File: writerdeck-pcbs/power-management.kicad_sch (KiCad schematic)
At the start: 36 parts, among them J1 5000mAh 3.7V LiPo, J3 5000mAh 3.7V LiPo, U2 BQ25792RQMR

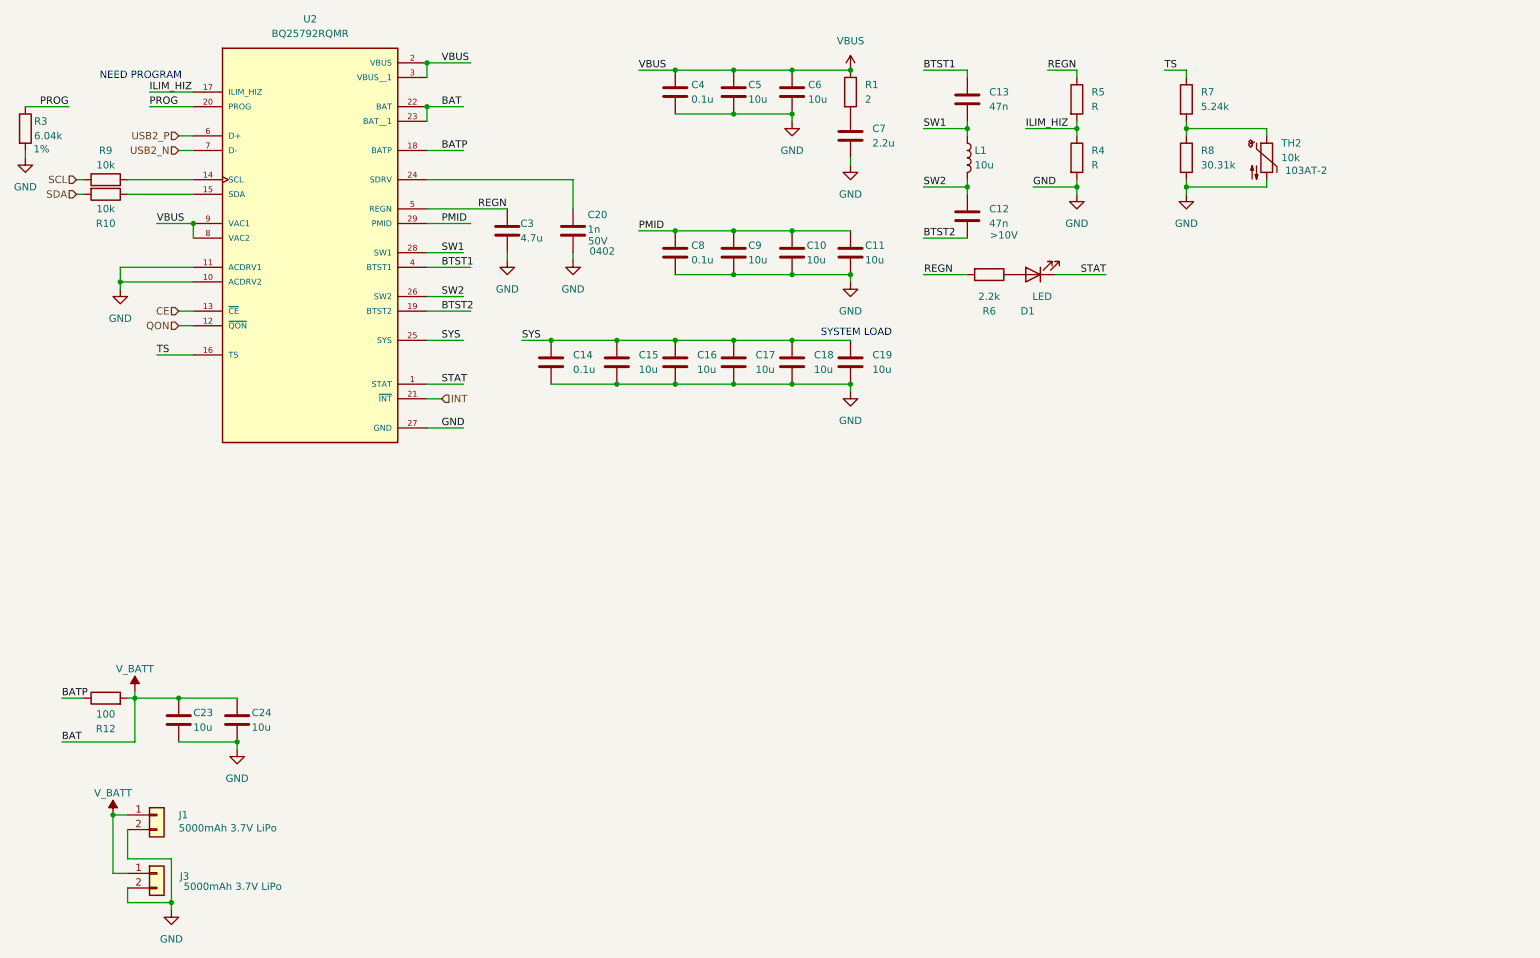
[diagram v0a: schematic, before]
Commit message: power management done
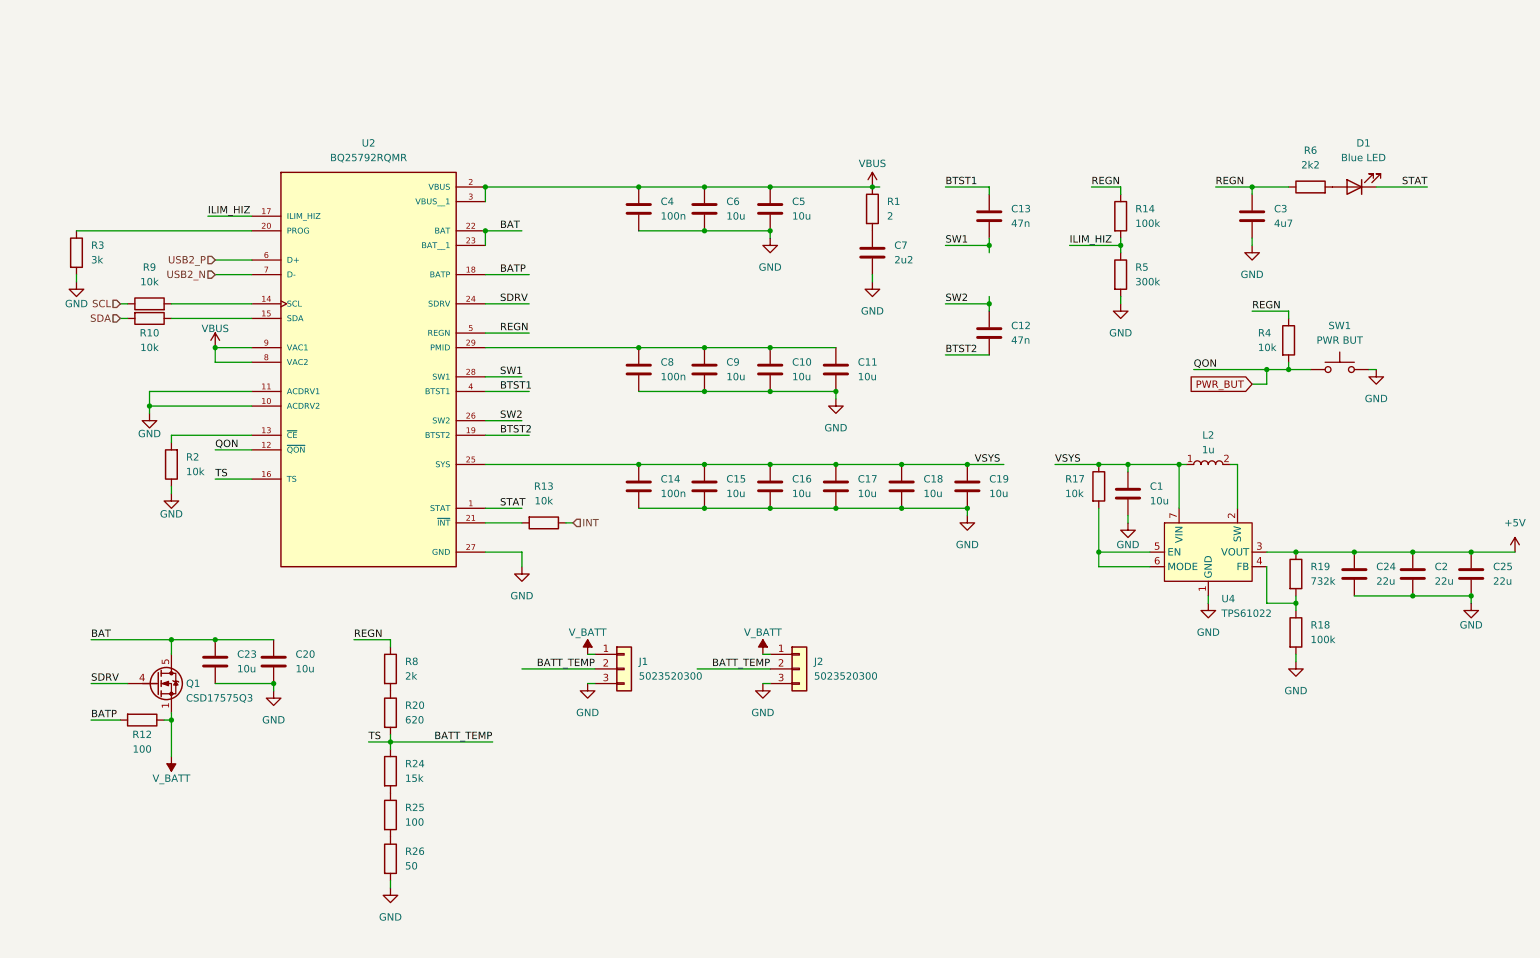
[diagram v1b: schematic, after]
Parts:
- removed C10, C11, C15, C16, C17, C18, C19, C23, C24, C5, C6, C9: 10u, symbol Device:C
- removed C12, C13: 47n, symbol Device:C
- removed C14, C4, C8: 0.1u, symbol Device:C
- removed C20: 1n, symbol Device:C
- removed C3: 4.7u, symbol Device:C
- removed C7: 2.2u, symbol Device:C
- removed D1: LED, symbol Device:LED
- removed J1, J3: 5000mAh 3.7V LiPo, symbol Connector_Generic:Conn_01x02
- removed L1: 10u, symbol Device:L
- removed R1: 2, symbol Device:R
- removed R10, R9: 10k, symbol Device:R
- removed R12: 100, symbol Device:R
- removed R3: 6.04k, symbol Device:R
- removed R4, R5: R, symbol Device:R
- removed R6: 2.2k, symbol Device:R
- removed R7: 5.24k, symbol Device:R
- removed R8: 30.31k, symbol Device:R
- removed TH2: 10k, symbol Device:Thermistor_NTC
- added C1, C10, C11, C15, C16, C17, C18, C19, C20, C23, C5, C6, C9: 10u, Capacitor_SMD:C_0603_1608Metric, symbol ZF_common:10u 10% 0603 Capacitor
- added C12, C13: 47n, Capacitor_SMD:C_0603_1608Metric, symbol ZF_common:47n 5% 0603 Capacitor
- added C14, C4, C8: 100n, Capacitor_SMD:C_0603_1608Metric, symbol ZF_common:100n 5% 0603 Capacitor
- added C2, C24, C25: 22u, Capacitor_SMD:C_0603_1608Metric, symbol ZF_common:22u 10% 0603 Capacitor
- added C3: 4u7, Capacitor_SMD:C_0603_1608Metric, symbol ZF_common:4u7 10% 0603 Capacitor
- added C7: 2u2, Capacitor_SMD:C_0603_1608Metric, symbol ZF_common:2u2 10% 0603 Capacitor
- added D1: Blue LED, LED_SMD:LED_0805_2012Metric, symbol ZF_common:0805 Blue LED
- added J1, J2: 5023520300, ZF_common:5023520300, symbol ZF_common:5023520300
- added L2: 1u, ZF_common:XFL4020-102MEC, symbol ZF_common:1uH XFL4020-102MEC
- added Q1: CSD17575Q3, Package_TO_SOT_SMD:TDSON-8-1, symbol Transistor_FET:CSD17570Q5B
- added R1: 2, Resistor_SMD:R_0603_1608Metric, symbol ZF_common:2 1% 0603 Resistor
- added R10, R13, R17, R2, R4, R9: 10k, Resistor_SMD:R_0603_1608Metric, symbol ZF_common:10k 1% 0603 Resistor
- added R12, R25: 100, Resistor_SMD:R_0603_1608Metric, symbol ZF_common:100 0.1% 0603 Resistor
- added R14, R18: 100k, Resistor_SMD:R_0603_1608Metric, symbol ZF_common:100k 1% 0603 Resistor
- added R19: 732k, Resistor_SMD:R_0603_1608Metric, symbol ZF_common:732k 1% 0603 Resistor
- added R20: 620, Resistor_SMD:R_0603_1608Metric, symbol ZF_common:620 1% 0603 Resistor
- added R24: 15k, Resistor_SMD:R_0603_1608Metric, symbol ZF_common:15k 1% 0603 Resistor
- added R26: 50, Resistor_SMD:R_0603_1608Metric, symbol ZF_common:50 0.1% 0603 Resistor
- added R3: 3k, Resistor_SMD:R_0603_1608Metric, symbol ZF_common:3k 1% 0603 Resistor
- added R5: 300k, Resistor_SMD:R_0603_1608Metric, symbol ZF_common:300k 1% 0603 Resistor
- added R6: 2k2, Resistor_SMD:R_0603_1608Metric, symbol ZF_common:2k2 1% 0603 Resistor
- added R8: 2k, Resistor_SMD:R_0603_1608Metric, symbol ZF_common:2k 1% 0603 Resistor
- added SW1: PWR BUT, symbol Switch:SW_Push
- added U4: TPS61022, Package_DFN_QFN:Texas_RWU0007A_VQFN-7_2x2mm_P0.5mm, symbol Converter_DCDC:TPS61022
- U2: DKN 296-BQ25792RQMRCT-ND -> (none); LCSCN (none) -> C2862876; MFR (none) -> Texas Instruments
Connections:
- net BATP: now also R12.2
- net BTST1: now also C13.1
- net BTST2: now also C12.2
- net GND: now also C1.2, C10.2, C11.2, C14.2, C15.2, C16.2, C17.2, C18.2, C19.2, C2.2, C20.2, C23.2, C24.2, C25.2, C3.2, C4.2, C5.2, C6.2, C7.2, C8.2, C9.2, J1.3 (Pin_3), J2.3 (Pin_3), R18.2, R2.1, R26.2, R3.2, R5.2, SW1.2, U4.1 (GND)
- net ILIM_HIZ: now also R14.2, R5.1
- net INT: now also R13.1; no longer U2.21 (~{INT})
- net REGN: now also C3.1, R14.1, R4.1, R6.1, R8.1
- net SCL: now also R9.1
- net SDA: now also R10.2
- net STAT: now also D1.1 (K)
- net SW1: now also C13.2
- net SW2: now also C12.1
- net VBUS: now also C4.1, C5.1, C6.1, R1.1
- net V_BATT: now also J1.1 (Pin_1), J2.1 (Pin_1), Q1.1 (S), Q1.2 (S), Q1.3 (S), R12.1; no longer U2.22 (BAT), U2.23 (BAT__1)
- net at U2.14 (SCL): now also R9.2
- net at U2.15 (SDA): now also R10.1
- net SDRV: now reaches U2.24 (SDRV)
- net SDRV: now also Q1.4 (G)
- net CE: no longer names the net of U2.13 (~{CE})
- net CE: now also R2.2
- net PMID: no longer names the net of U2.29 (PMID)
- net PMID: now also C10.1, C11.1, C8.1, C9.1
- net PROG: no longer names the net of U2.20 (PROG)
- net PROG: now also R3.1
- net QON renamed PWR_BUT
- net PWR_BUT: now also R4.2, SW1.1
- net SYS renamed VSYS
- net VSYS: now also C1.1, C14.1, C15.1, C16.1, C17.1, C18.1, C19.1, L2.1, R17.1, U4.7 (VIN)
- net TS renamed BATT_TEMP
- net BATT_TEMP: now also J1.2 (Pin_2), J2.2 (Pin_2), R20.2, R24.1
- new net: D1.2 (A), R6.2
- new net: R25.2, R26.1
- new net: R13.2, U2.21 (~{INT})
- new net: L2.2, U4.2 (SW)
- new net: R18.1, R19.2, U4.4 (FB)
- new net: R17.2, U4.5 (EN), U4.6 (MODE)
- new net: R20.1, R8.2
- new net: R24.2, R25.1
- new net: C7.1, R1.2
- new net +5V: C2.1, C24.1, C25.1, R19.1, U4.3 (VOUT)
- new net BAT: C20.1, C23.1, Q1.5 (D), U2.22 (BAT), U2.23 (BAT__1)
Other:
- note removed: "NEED PROGRAM"
- note removed: "SYSTEM LOAD"
- moved on the sheet: U2
